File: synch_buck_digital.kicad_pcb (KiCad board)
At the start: 4 copper layers, 60 x 60 mm, 48 parts, among them U1 BSC066N06NSATMA1, U2 BSC066N06NSATMA1, U3 INA241A3IDDFR

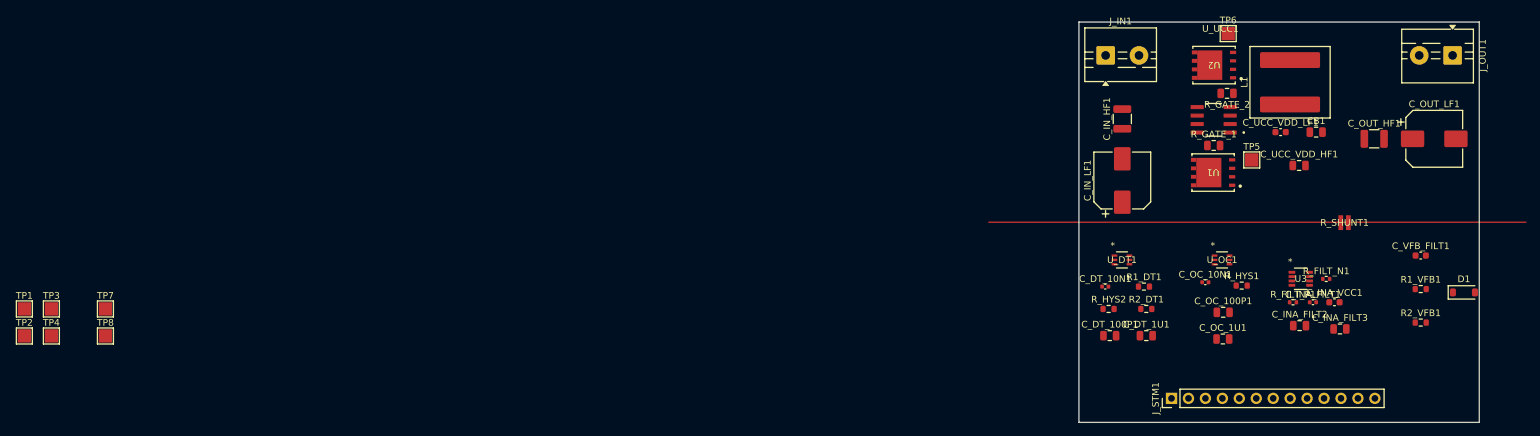
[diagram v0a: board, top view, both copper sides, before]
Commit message: update
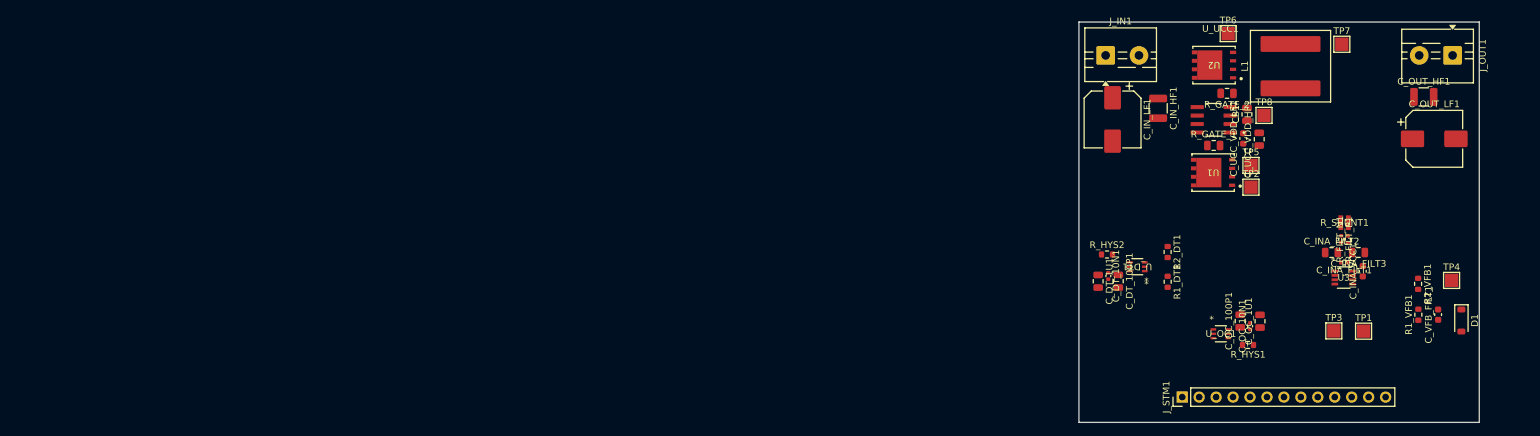
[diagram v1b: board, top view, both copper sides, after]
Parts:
- moved TP4 210.0 mm to (235.8, 92.7)
- moved TP1 200.7 mm to (222.7, 100.3)
- moved TP3 192.2 mm to (218.2, 100.3)
- moved TP7 189.5 mm to (219.4, 57.3)
- moved TP2 185.2 mm to (205.8, 78.8)
- moved TP8 176.8 mm to (207.7, 68.0)
- moved C_INA_FILT2 12.0 mm to (217.9, 88.5)
- moved R_FILT_P1 11.9 mm to (219.3, 86.5), turned to -90 degrees
- moved C_INA_FILT3 11.8 mm to (221.9, 88.5), turned to 180 degrees
- moved U_OC1 11.1 mm to (201.3, 100.7)
- moved C_DT_1U1 10.9 mm to (182.9, 92.8), turned to -90 degrees
- moved CB1 10.7 mm to (205.2, 67.8), turned to 90 degrees
- moved C_OUT_HF1 9.73 mm to (231.7, 65.2)
- moved C_OC_10N1 9.40 mm to (205.7, 99.6), turned to 90 degrees
- moved C_IN_LF1 9.26 mm to (185.0, 68.6), turned to -90 degrees
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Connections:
- C_DT_100P1 pad 2: PGND -> SGND
- C_DT_10N1 pad 2: PGND -> SGND
- C_DT_1U1 pad 2: PGND -> SGND
- C_INA_FILT2 pad 1: PGND -> SGND
- C_INA_FILT3 pad 1: PGND -> SGND
- C_INA_VCC1 pad 2: PGND -> SGND
- C_OC_100P1 pad 2: PGND -> SGND
- C_OC_10N1 pad 2: PGND -> SGND
- C_OC_1U1 pad 2: PGND -> SGND
- C_VFB_FILT1 pad 1: PGND -> SGND
- D1 pad 2: PGND -> SGND
- J_STM1 pad 1: /PWM_LS -> /DT_REF
- J_STM1 pad 10: PGND -> SGND
- J_STM1 pad 11: PGND -> SGND
- J_STM1 pad 12: PGND -> SGND
- J_STM1 pad 13: PGND -> SGND
- J_STM1 pad 2: /V_FB -> /COMP_OUT
- J_STM1 pad 3: /DT_REF -> /PROT_OUT
- J_STM1 pad 5: /PROT_OUT -> /PWM_LS
- J_STM1 pad 6: /SENSE_OUT -> /PWM_HS
- J_STM1 pad 7: /PWM_HS -> /SENSE_OUT
- J_STM1 pad 8: /COMP_OUT -> /V_FB
- R1_DT1 pad 2: PGND -> SGND
- R1_VFB1 pad 1: PGND -> SGND
- R_HYS1 pad 1: PGND -> SGND
- R_HYS2 pad 1: PGND -> SGND
- TP1 pad 1: PGND -> SGND
- U3 pad 2: PGND -> SGND
- U3 pad 3: PGND -> SGND
- U3 pad 4: PGND -> SGND
- U3 pad 7: PGND -> SGND
- U_DT1 pad 2: PGND -> SGND
- U_OC1 pad 2: PGND -> SGND
- U_UCC1 pad 7: PGND -> SGND
